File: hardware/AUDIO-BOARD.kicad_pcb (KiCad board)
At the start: 2 copper layers, 66 x 46 mm, 88 parts, among them J1 CON_USB_GCT_USB4105_REVA, J2 STLINK, J3 SD-CARD-MEM2051-00-195-00-A, J4 SJ-3523-SMT-TR, J5 MIC, J6 CON_USB_GCT_USB4105_REVA, J7 BATT, M1 MNT, M2 MNT, M3 MNT, M4 MNT, SW1 RST, U1 STM32F446RETx, U10 TPS2116, U2 D-ESD-PESD2ETH-AD, U3 TSOP38G36, U4 CS42L51-CNZ, U5 MCP73831-2-OT, U6 TLV73333PDBV, U7 NCP163ASN250T1G, U8 AP22652W6-7, U9 TPS613222ADBV, Y1 8MHz

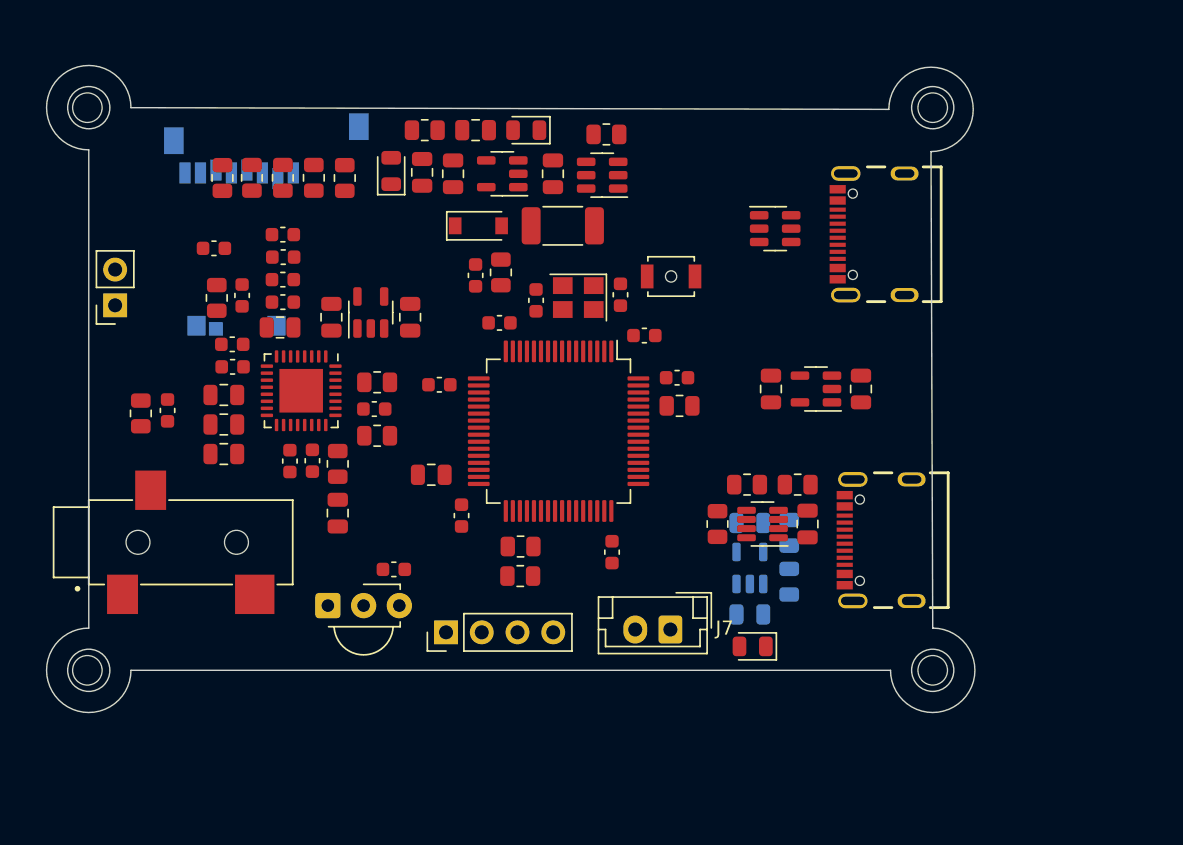
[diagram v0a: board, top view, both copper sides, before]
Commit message: Update the PCB routing
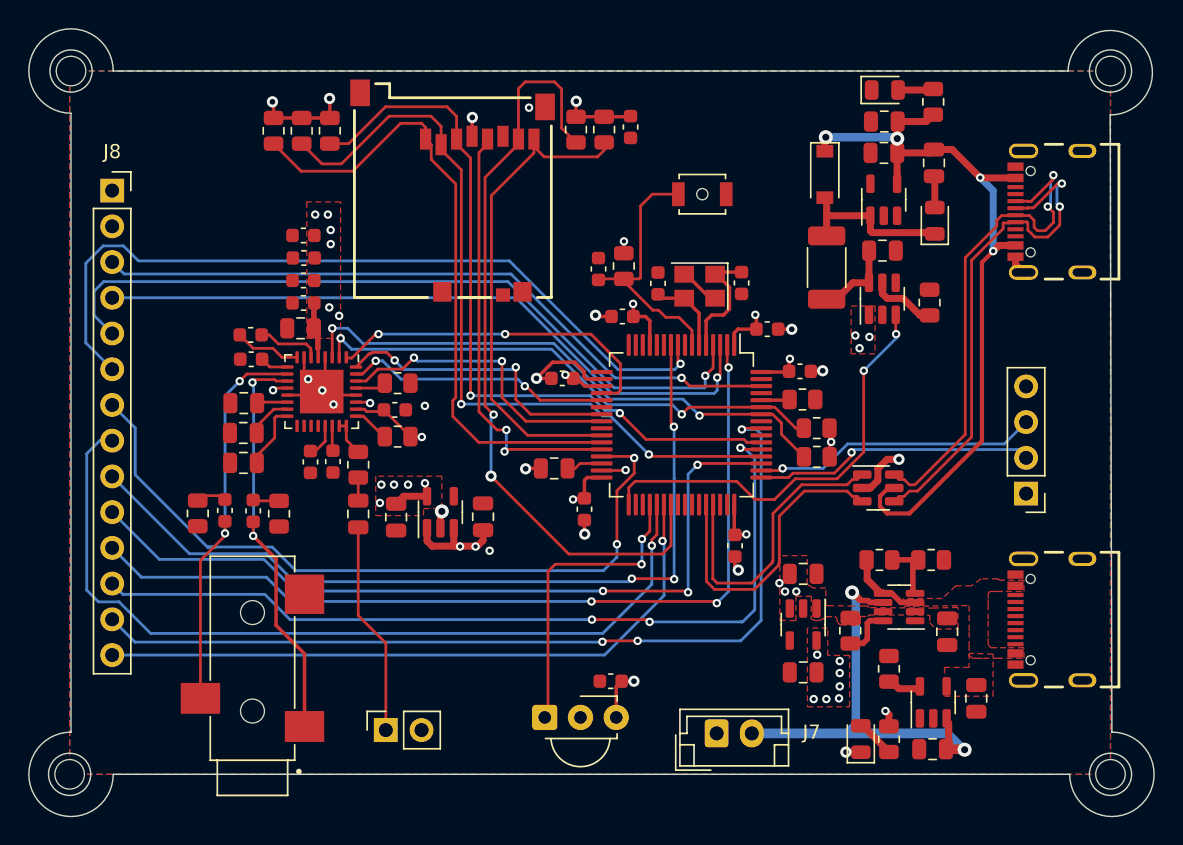
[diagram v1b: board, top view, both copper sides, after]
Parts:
- added J8: TFT TOUCH SCREEN, Connector_PinSocket_2.54mm:PinSocket_1x14_P2.54mm_Vertical, F.Cu at (108.7, 59.9)
- C29, C30, J3, R15, R16, U5: moved to F.Cu
- moved J2 42.4 mm to (173.6, 81.4), turned to 180 degrees
- moved R21 36.2 mm to (167.0, 53.6), turned to 90 degrees
- moved J5 35.8 mm to (128.1, 98.2), turned to 90 degrees
- moved D3 35.6 mm to (163.6, 52.7), turned to 0 degrees
- moved C38 33.1 mm to (163.6, 55.0), turned to 180 degrees
- moved C36 32.7 mm to (167.1, 57.9), turned to 90 degrees
- moved C12 30.8 mm to (145.5, 55.4), turned to -90 degrees
- moved C37 30.7 mm to (163.5, 57.2), turned to 180 degrees
- moved R18 29.8 mm to (167.1, 62.0), turned to 90 degrees
- moved U9 27.2 mm to (163.5, 60.5), turned to 90 degrees
- moved R17 25.9 mm to (166.8, 67.9), turned to 90 degrees
- moved D2 24.9 mm to (159.3, 58.7), turned to -90 degrees
- moved C35 24.1 mm to (163.4, 64.2), turned to 0 degrees
- moved R6 22.7 mm to (158.8, 78.8)
- moved R4 22.7 mm to (158.8, 76.8)
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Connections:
- J1 pad A4/B9: /USB_POWER -> /USB_OTG_VBUS
- J1 pad B4/A9: /USB_POWER -> /USB_OTG_VBUS
- U1 pad 10: unconnected-(U1-Pad10) -> SPI2_MISO_PC2
- U1 pad 2: unconnected-(U1-Pad2) -> SPI3_nCS_PC13
- U1 pad 29: unconnected-(U1-Pad29) -> SPI2_SCK_PB10
- U1 pad 3: unconnected-(U1-Pad3) -> LCD_RST_PC14
- U1 pad 37: unconnected-(U1-Pad37) -> LCD_LED_PC6
- U1 pad 38: unconnected-(U1-Pad38) -> LCD_T_IRQ_PC7
- U1 pad 4: unconnected-(U1-Pad4) -> LCD_DC_PC15
- U1 pad 51: unconnected-(U1-Pad51) -> SPI3_SCK_PC10
- U1 pad 53: unconnected-(U1-Pad53) -> SPI3_MOSI_PC12
- U1 pad 56: unconnected-(U1-Pad56) -> SPI3_MISO_PB4
- U1 pad 62: unconnected-(U1-Pad62) -> SPI2_nCS_PB9
- U1 pad 9: unconnected-(U1-Pad9) -> SPI2_MOSI_PC1
- U2 pad 5: /USB_POWER -> /USB_OTG_VBUS
- U8 pad 3: /PowerSupply/USB_OTG_EN -> /USB_OTG_EN
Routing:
- net SPI3_MISO_PB4: track 0.00 -> 63.6 mm, vias 0 -> 3
- net SPI3_nCS_PC13: track 0.00 -> 63.4 mm, vias 0 -> 3
- net SPI3_MOSI_PC12: track 0.00 -> 60.8 mm, vias 0 -> 3
- net LCD_LED_PC6: track 0.00 -> 60.6 mm, vias 0 -> 1
- net SPI2_MISO_PC2: track 0.00 -> 59.9 mm, vias 0 -> 3
- net SPI3_SCK_PC10: track 0.00 -> 57.2 mm, vias 0 -> 3
- net SPI2_MOSI_PC1: track 0.00 -> 56.3 mm, vias 0 -> 1
- net SD_D3_PC11: track 0.00 -> 55.4 mm, vias 0 -> 2
- net /USB_OTG_VBUS: track 0.00 -> 55.4 mm, vias 0 -> 4
- net SD_D0_PC8: track 0.00 -> 54.8 mm, vias 0 -> 2
- net LCD_DC_PC15: track 0.00 -> 53.6 mm, vias 0 -> 1
- net SPI2_SCK_PB10: track 0.00 -> 53.6 mm, vias 0 -> 2
- net SD_CMD_PD2: track 0.00 -> 52.7 mm, vias 0 -> 2
- net SPI2_nCS_PB9: track 0.00 -> 49.8 mm, vias 0 -> 1
- net LCD_RST_PC14: track 0.00 -> 49.2 mm, vias 0 -> 1
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- added copper zone on F.Cu, net +2V5
- added copper zone on In2.Cu, net +2V5
- added copper zone on F.Cu, net +3.3V
- added copper zone on In2.Cu, net +3.3V
- added copper zone on F.Cu, net /PowerSupply/MAIN_PWR
- added copper zone on In2.Cu, net /PowerSupply/MAIN_PWR
- added copper zone on B.Cu, net GND
- added copper zone on F.Cu, net GND
- added copper zone on In1.Cu, net GND
- added copper zone on F.Cu, net VBUS
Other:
- board size 66 x 46 mm -> 80 x 56 mm
- copper layers 2 -> 4
